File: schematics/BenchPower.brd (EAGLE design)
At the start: 80 x 67 mm, 28 parts, among them U1 V_REG_317SINK, X2 9090-4R

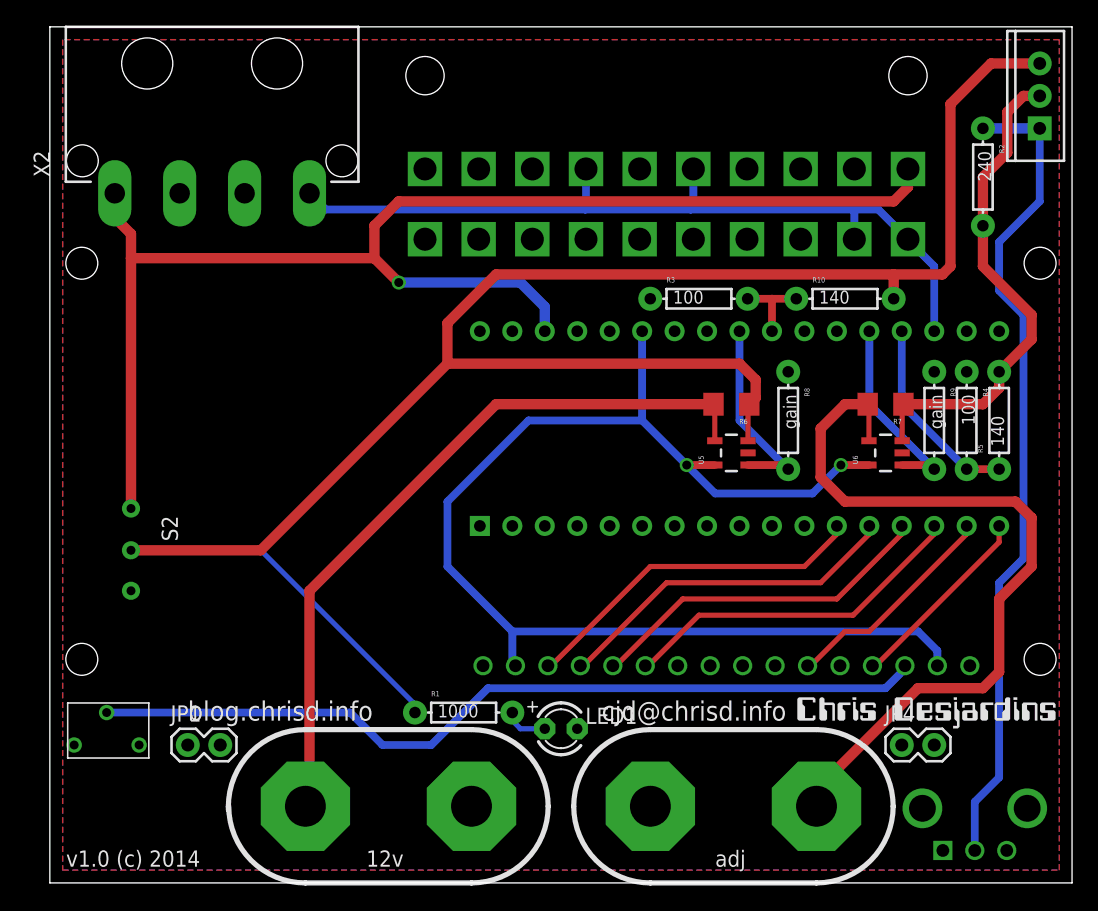
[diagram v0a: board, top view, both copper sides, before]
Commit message: Updates for rev 2
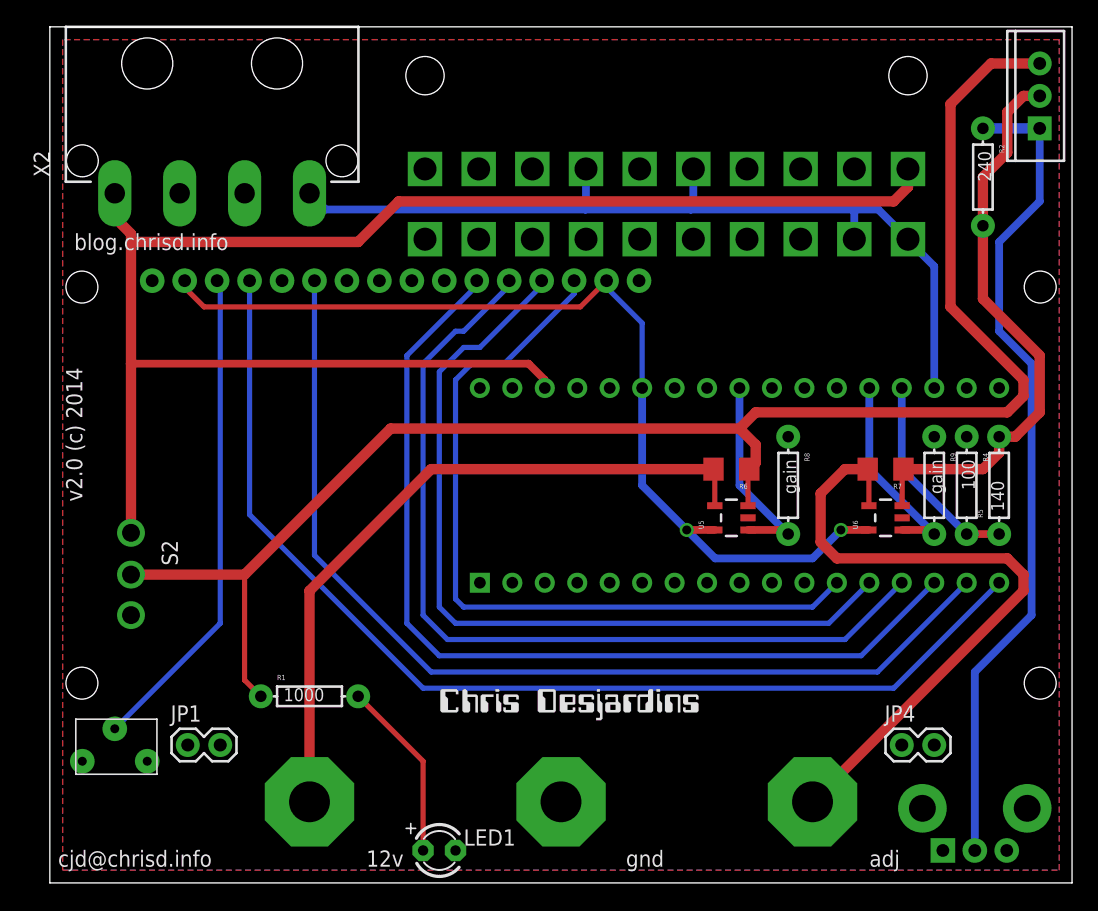
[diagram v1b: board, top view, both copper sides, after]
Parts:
- removed R10: 140, SparkFun-Passives:AXIAL-0.3
- removed R3: 100, SparkFun-Passives:AXIAL-0.3
- removed U$6: BINDINGPOST, desjardins:BINDINGPOST
- moved U$3 27.9 mm to (30.5, 13.3)
- moved LED1 13.5 mm to (30.5, 2.54)
- moved R1 12.1 mm to (20.3, 14.6)
- moved U$5 7.01 mm to (40.0, 6.35)
- moved R6 5.08 mm to (53.3, 32.4)
- moved R7 5.08 mm to (65.4, 32.4)
- moved R4 5.08 mm to (71.8, 31.1)
- moved R5 5.08 mm to (74.3, 31.1)
- moved R8 5.08 mm to (57.8, 31.1)
- moved R9 5.08 mm to (69.2, 31.1)
- moved U5 5.08 mm to (53.3, 28.6)
- moved U6 5.08 mm to (65.4, 28.6)
- moved U$2 4.45 mm to (78.1, 22.2)
- moved S2 1.91 mm to (6.35, 24.1)
- moved U$4 1.87 mm to (40.0, 31.1), turned to 0 degrees
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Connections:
- net 12VHDRSW: no longer R10.P$2
- net 12VHDRTAP: no longer R10.P$1, R3.P$2
- net GND: no longer R3.P$1, U$6.P$1
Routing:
- net LCD_RS: track 15.2 -> 86.0 mm
- net LCD_EN: track 17.4 -> 79.2 mm
- net LCD_DB4: track 27.5 -> 73.8 mm
- net LCD_DB5: track 27.5 -> 69.4 mm
- net LCD_DB6: track 27.5 -> 65.1 mm
- net LCD_DB7: track 27.5 -> 61.1 mm
- net 12VHDRSW: track 155.6 -> 126.0 mm
- net LCD_CONTRAST: track 66.2 -> 38.6 mm
- net 5VARDU: track 98.2 -> 75.4 mm
- net 12VHDR: track 108.0 -> 124.7 mm, vias 1 -> 0
- net N$1: track 3.44 -> 14.2 mm
- net AMPS12VREG: track 61.5 -> 52.7 mm
- net 12VREG: track 39.0 -> 45.3 mm
- net 12VHDRTAP: track 6.35 -> 0.00 mm
- net 5VHDR: track 65.2 -> 69.6 mm
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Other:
- board text added: "gnd"
- board text added: "v2.0 (c) 2014"
- board text removed: "v1.0 (c) 2014"
